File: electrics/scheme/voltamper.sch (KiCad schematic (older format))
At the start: 20 parts

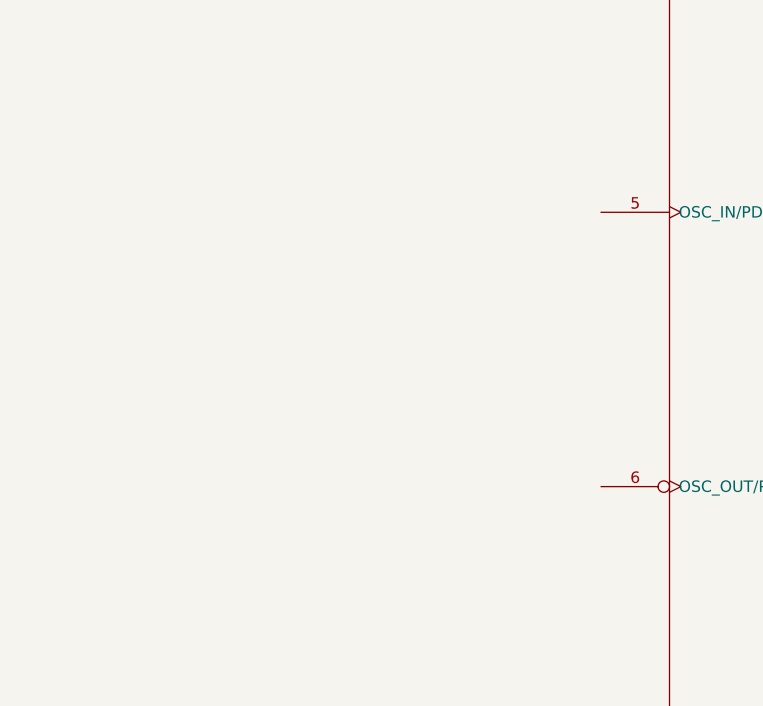
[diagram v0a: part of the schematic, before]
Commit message: a
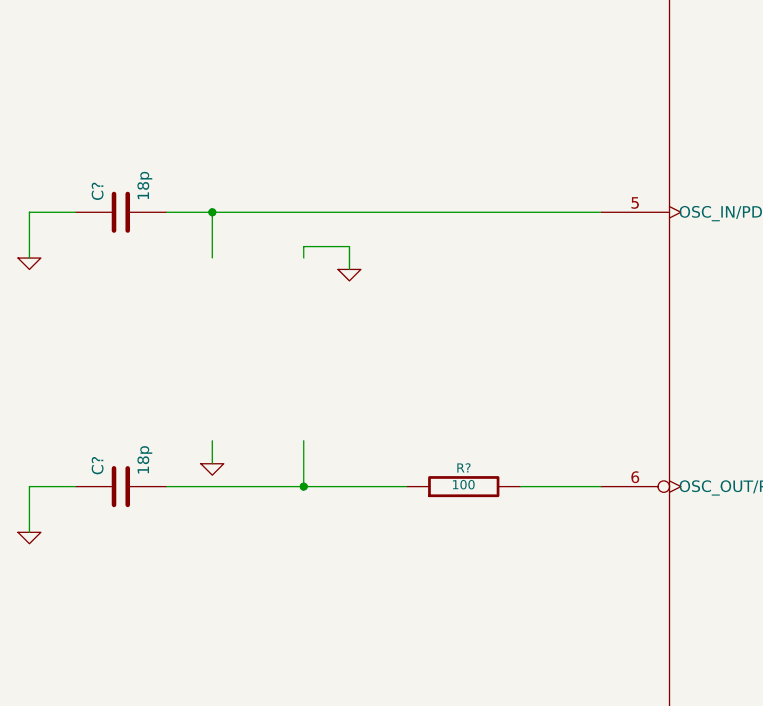
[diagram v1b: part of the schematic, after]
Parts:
- added C? (x2): 18p, symbol C
- added R?: 100, ~, symbol R
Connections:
- wire segments 82 -> 95
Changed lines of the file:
@@
 	1    0    0    -1
 $EndComp
+$Comp
+L GND #PWR?
+U 1 1 5480CD20
+P 1200 5700
+F 0 "#PWR?" H 1200 5700 30  0001 C CNN
+F 1 "GND" H 1200 5630 30  0001 C CNN
+F 2 "" H 1200 5700 60  0001 C CNN
+F 3 "" H 1200 5700 60  0001 C CNN
+	1    1200 5700
+	1    0    0    -1
+$EndComp
+$Comp
+L C C?
+U 1 1 5480CD26
+P 1600 6700
+F 0 "C?" H 1650 6800 50  0000 L CNN
+F 1 "18p" H 1650 6600 50  0000 L CNN
+F 2 "" H 1600 6700 60  0001 C CNN
+F 3 "" H 1600 6700 60  0001 C CNN
+	1    1600 6700
+	0    -1   -1   0
+$EndComp
+$Comp
+L C C?
+U 1 1 5480CD2C
+P 1600 5500
+F 0 "C?" H 1650 5600 50  0000 L CNN
+F 1 "18p" H 1650 5400 50  0000 L CNN
+F 2 "" H 1600 5500 60  0001 C CNN
+F 3 "" H 1600 5500 60  0001 C CNN
+	1    1600 5500
+	0    -1   -1   0
+$EndComp
+Wire Wire Line
+	2400 6500 2400 6700
+Wire Wire Line
+	1800 6700 2850 6700
+Wire Wire Line
+	2000 5700 2000 5500
+Wire Wire Line
+	1800 5500 3700 5500
+Wire Wire Line
+	1400 5500 1200 5500
+Wire Wire Line
+	1200 5500 1200 5700
+Wire Wire Line
+	1400 6700 1200 6700
+Wire Wire Line
+	1200 6700 1200 6900
+$Comp
+L GND #PWR?
+U 1 1 5480CD40
+P 1200 6900
+F 0 "#PWR?" H 1200 6900 30  0001 C CNN
+F 1 "GND" H 1200 6830 30  0001 C CNN
+F 2 "" H 1200 6900 60  0001 C CNN
+F 3 "" H 1200 6900 60  0001 C CNN
+	1    1200 6900
+	1    0    0    -1
+$EndComp
+Connection ~ 2000 5500
+Connection ~ 2400 6700
+$Comp
+L R R?
+U 1 1 5480CD4A
+P 3100 6700
+F 0 "R?" V 3180 6700 40  0000 C CNN
+F 1 "100" V 3107 6701 40  0000 C CNN
+F 2 "~" V 3030 6700 30  0000 C CNN
+F 3 "~" H 3100 6700 30  0000 C CNN
+	1    3100 6700
+	0    -1   -1   0
+$EndComp
+Wire Wire Line
+	2400 5700 2400 5650
+Wire Wire Line
+	2400 5650 2600 5650
+Wire Wire Line
+	2600 5650 2600 5750
+$Comp
+L GND #PWR?
+U 1 1 5480CD54
+P 2600 5750
+F 0 "#PWR?" H 2600 5750 30  0001 C CNN
+F 1 "GND" H 2600 5680 30  0001 C CNN
+F 2 "" H 2600 5750 60  0001 C CNN
+F 3 "" H 2600 5750 60  0001 C CNN
+	1    2600 5750
+	1    0    0    -1
+$EndComp
+Wire Wire Line
+	2000 6500 2000 6600
+$Comp
+L GND #PWR?
+U 1 1 5480CD5B
+P 2000 6600
+F 0 "#PWR?" H 2000 6600 30  0001 C CNN
+F 1 "GND" H 2000 6530 30  0001 C CNN
+F 2 "" H 2000 6600 60  0001 C CNN
+F 3 "" H 2000 6600 60  0001 C CNN
+	1    2000 6600
+	1    0    0    -1
+$EndComp
+Wire Wire Line
+	3350 6700 3700 6700
 $EndSCHEMATC
